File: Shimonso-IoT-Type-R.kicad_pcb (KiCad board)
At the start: 4 copper layers, 85 x 54 mm, 116 parts, among them CON1 96Boards_HS_connector, CON2 96Boards_LS_connector, CON3 microUSB_CONSOLE, CON4 CONN_01X15, CON5 CONN_01X15, Q1 S8050, SW1 RST, U1 FT230X, U10 PCA9306DC1, U11 bm1422gmv, U12 BU9873, U13 rpr-0521rs, U14 bh1745nuc, U15 ADS1115, U16 MC-306_32.768K-E3, U17 BD1020HFV, U18 ML8511A, U2 BD33GC0WEFJ, U3 BD18GC0WEFJ, U4 SN74AVC4T245, U5 PCA9306DC1, U6 PCA9306DC1, U7 bd7411g, U8 kx022-1020, U9 bm1383glv

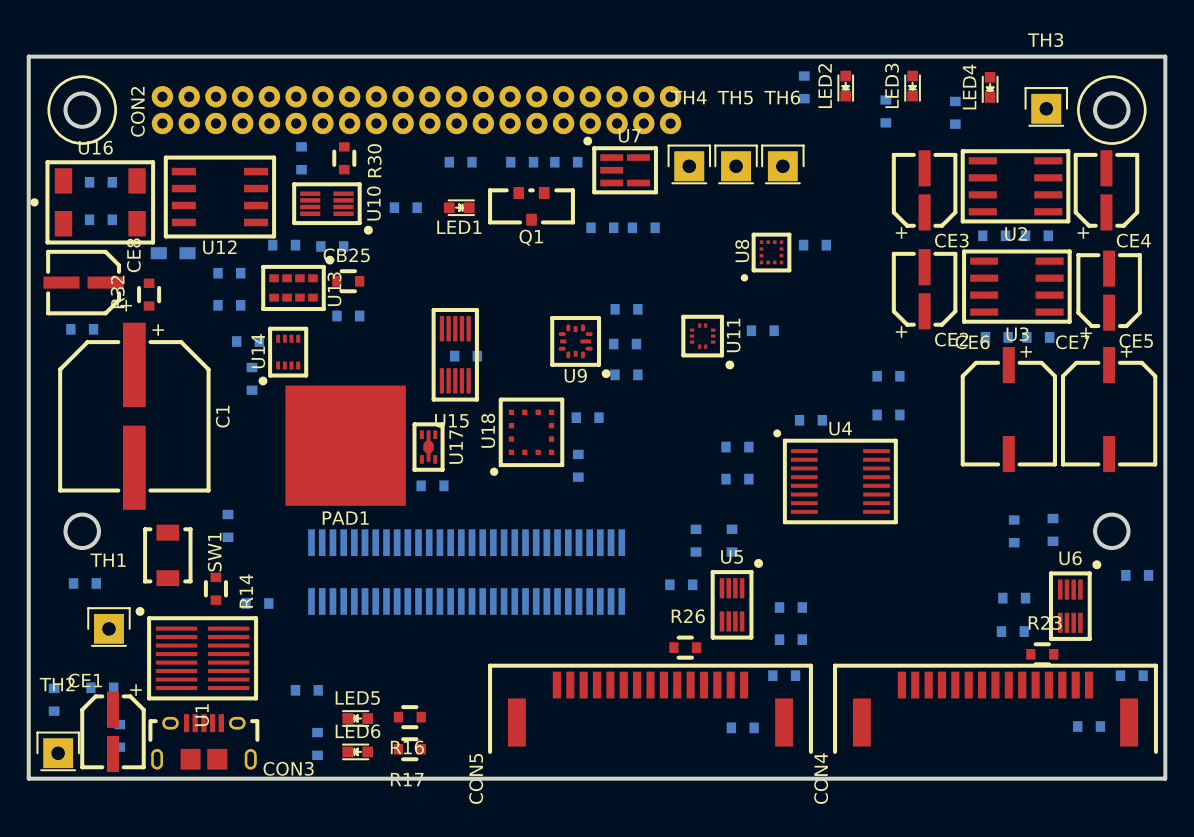
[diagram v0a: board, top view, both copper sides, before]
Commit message: modified
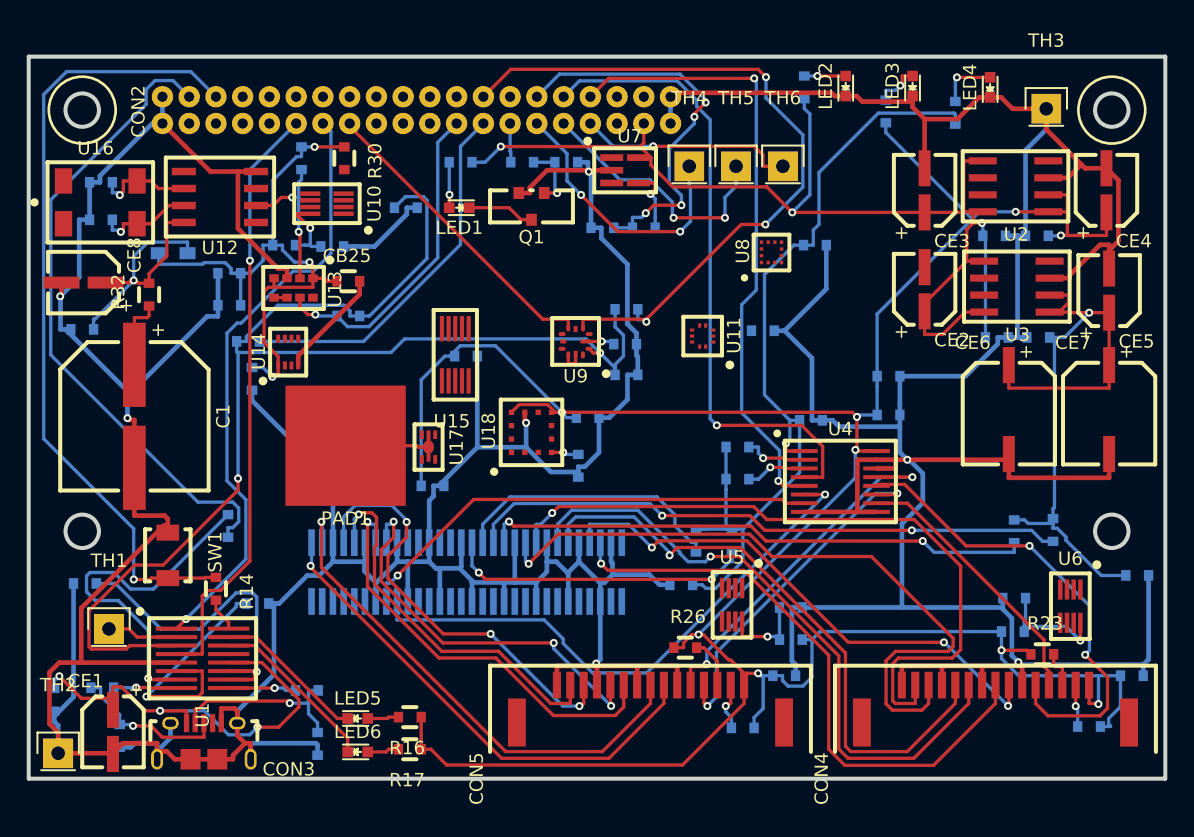
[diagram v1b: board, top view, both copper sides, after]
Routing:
- net GND: track 0.00 -> 569.9 mm, vias 0 -> 7
- net /3V3: track 0.00 -> 255.4 mm, vias 0 -> 12
- net /1V8: track 0.00 -> 212.8 mm, vias 0 -> 4
- net /5V: track 0.00 -> 85.1 mm, vias 0 -> 3
- net /EXP_RSTOUT_N: track 0.00 -> 59.6 mm, vias 0 -> 1
- net /BM1383GLV_INT: track 0.00 -> 54.5 mm, vias 0 -> 3
- net /CSI1_DATA0_N: track 0.00 -> 53.2 mm, vias 0 -> 1
- net /CSI1_DATA0_P: track 0.00 -> 51.8 mm, vias 0 -> 1
- net /PMU_PWRON_N: track 0.00 -> 48.3 mm
- net /CAM1_GPIO: track 0.00 -> 48.2 mm, vias 0 -> 1
- net /CSI1_DATA1_P: track 0.00 -> 47.8 mm, vias 0 -> 1
- net /CAM2_GPIO: track 0.00 -> 46.8 mm, vias 0 -> 2
- net /CSI1_DATA1_N: track 0.00 -> 45.4 mm, vias 0 -> 1
- net /UART3_TX: track 0.00 -> 45.1 mm, vias 0 -> 1
- net /UART3_RX: track 0.00 -> 45.0 mm, vias 0 -> 1
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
